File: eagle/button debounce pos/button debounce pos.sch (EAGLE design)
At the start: 21 parts, among them IC1 74LS14N, X1 MKDSN1,5/2-5,08, X2 MKDSN1,5/6-5,08

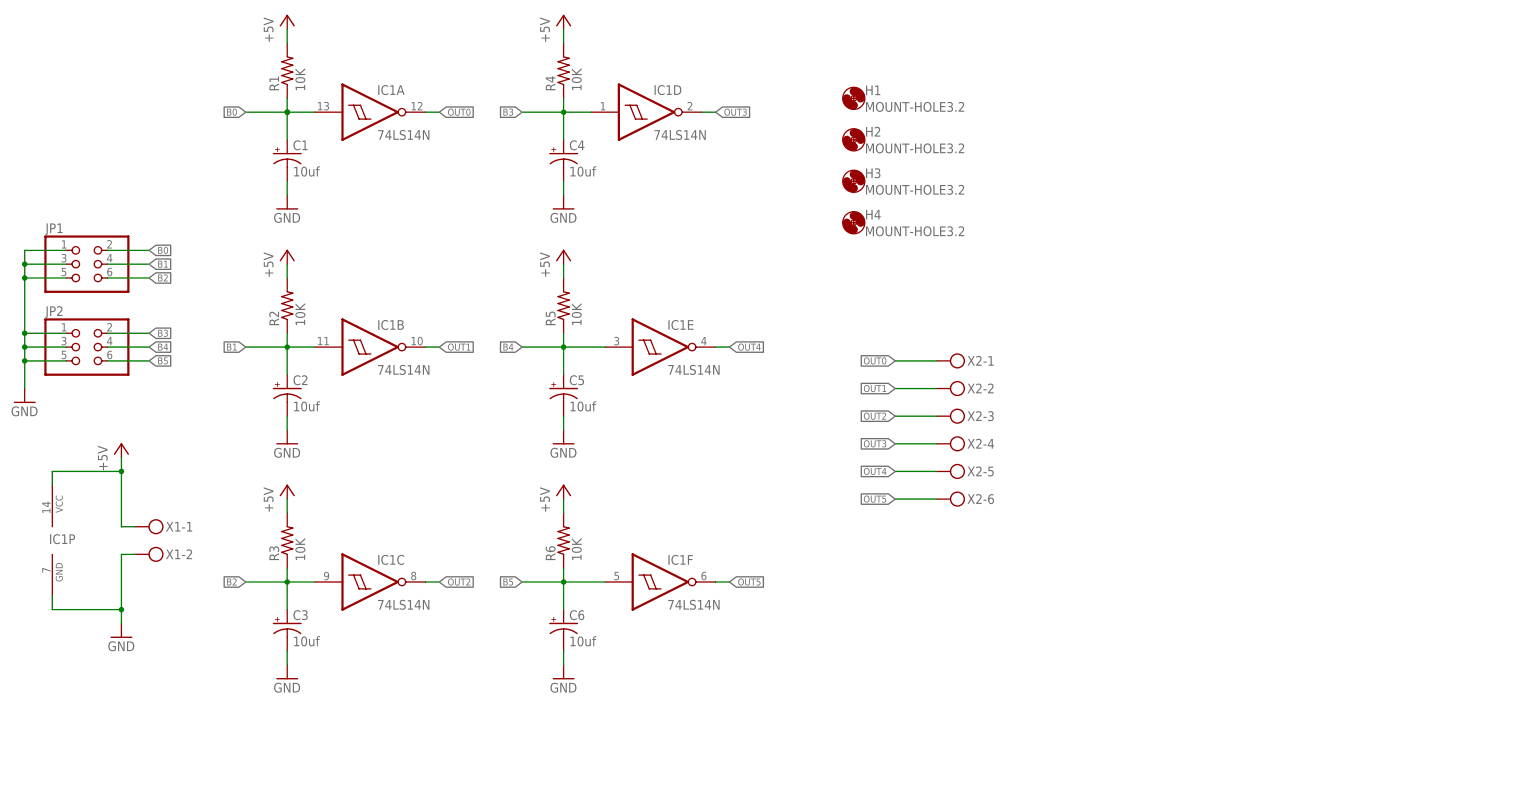
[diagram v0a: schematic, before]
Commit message: check in changes
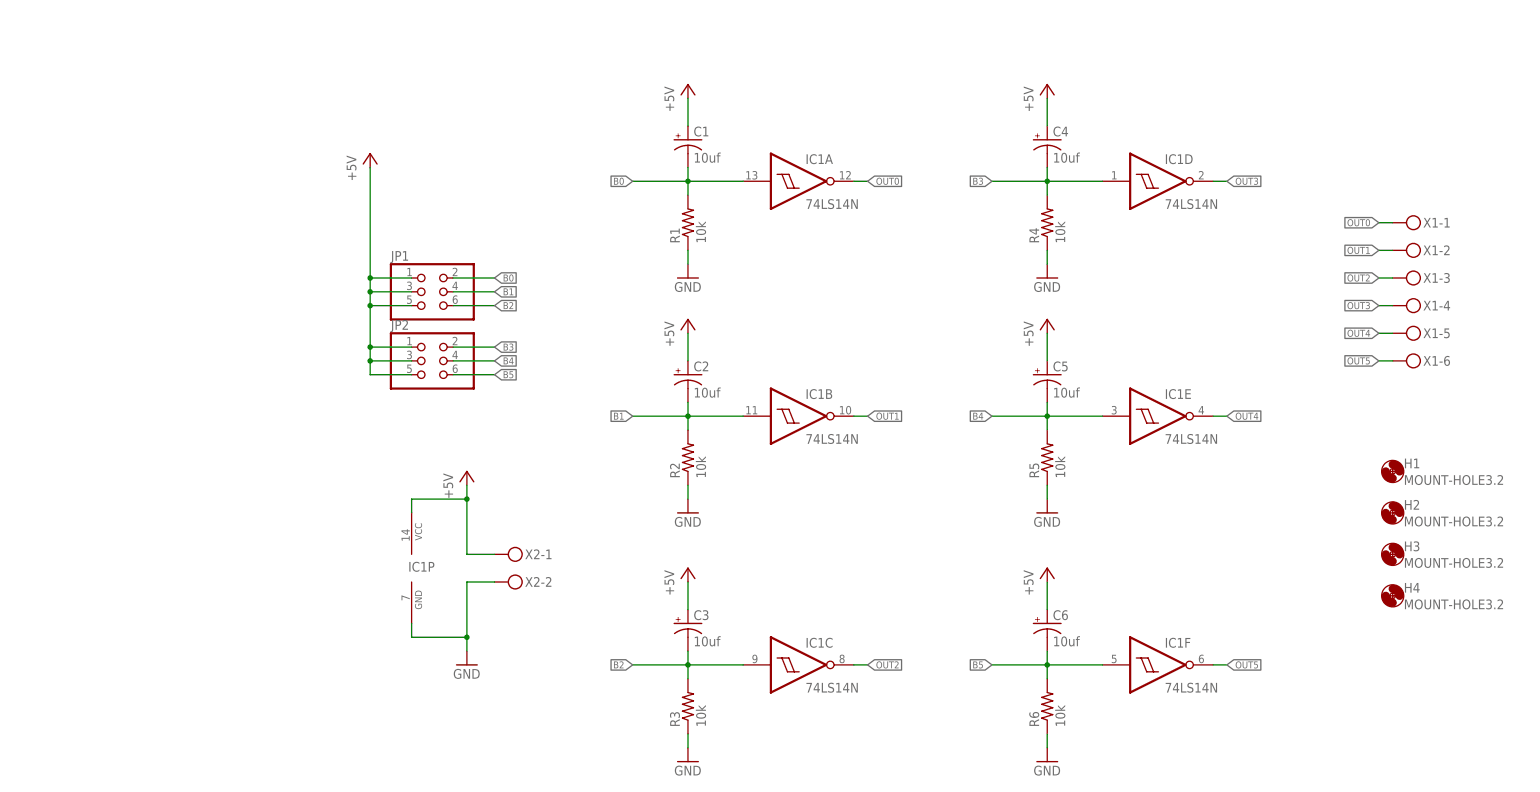
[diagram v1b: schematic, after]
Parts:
- R1, R2, R3, R4, R5, R6: value 10K -> 10k
- X1: value MKDSN1,5/2-5,08 -> MKDSN1,5/6-5,08; device con-phoenix-508:MKDSN1,5/2-5,08 -> con-phoenix-508:MKDSN1,5/6-5,08
- X2: value MKDSN1,5/6-5,08 -> MKDSN1,5/2-5,08; device con-phoenix-508:MKDSN1,5/6-5,08 -> con-phoenix-508:MKDSN1,5/2-5,08
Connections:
- net +5V: now also C1.+, C2.+, C3.+, C4.+, C5.+, C6.+, JP1.1, JP1.3, JP1.5, JP2.1, JP2.3, JP2.5, X2-1.KL; no longer R1.2, R2.2, R3.2, R4.2, R5.2, R6.2, X1-1.KL
- net B0: now also C1.-, R1.2; no longer C1.+, R1.1
- net B1: now also C2.-, R2.2; no longer C2.+, R2.1
- net B2: now also C3.-, R3.2; no longer C3.+, R3.1
- net B3: now also C4.-, R4.2; no longer C4.+, R4.1
- net B4: now also C5.-, R5.2; no longer C5.+, R5.1
- net B5: now also C6.-, R6.2; no longer C6.+, R6.1
- net GND: now also R1.1, R2.1, R3.1, R4.1, R5.1, R6.1, X2-2.KL; no longer C1.-, C2.-, C3.-, C4.-, C5.-, C6.-, JP1.1, JP1.3, JP1.5, JP2.1, JP2.3, JP2.5, X1-2.KL
- net OUT0: now also X1-1.KL; no longer X2-1.KL
- net OUT1: now also X1-2.KL; no longer X2-2.KL
- net OUT2: now also X1-3.KL; no longer X2-3.KL
- net OUT3: now also X1-4.KL; no longer X2-4.KL
- net OUT4: now also X1-5.KL; no longer X2-5.KL
- net OUT5: now also X1-6.KL; no longer X2-6.KL
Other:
- moved on the sheet: C1, C2, C3, C4, C5, C6, H1, H2, H3, H4, IC1A, IC1B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
